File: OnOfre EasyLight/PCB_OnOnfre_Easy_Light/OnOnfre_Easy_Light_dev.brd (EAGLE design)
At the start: 44.6 x 48 mm, 38 parts, among them J3Y S8050, K1 OMRON-G3MB-202P-SSR2, K2 OMRON-G3MB-202P-SSR2, U2 esp12, X1 4P

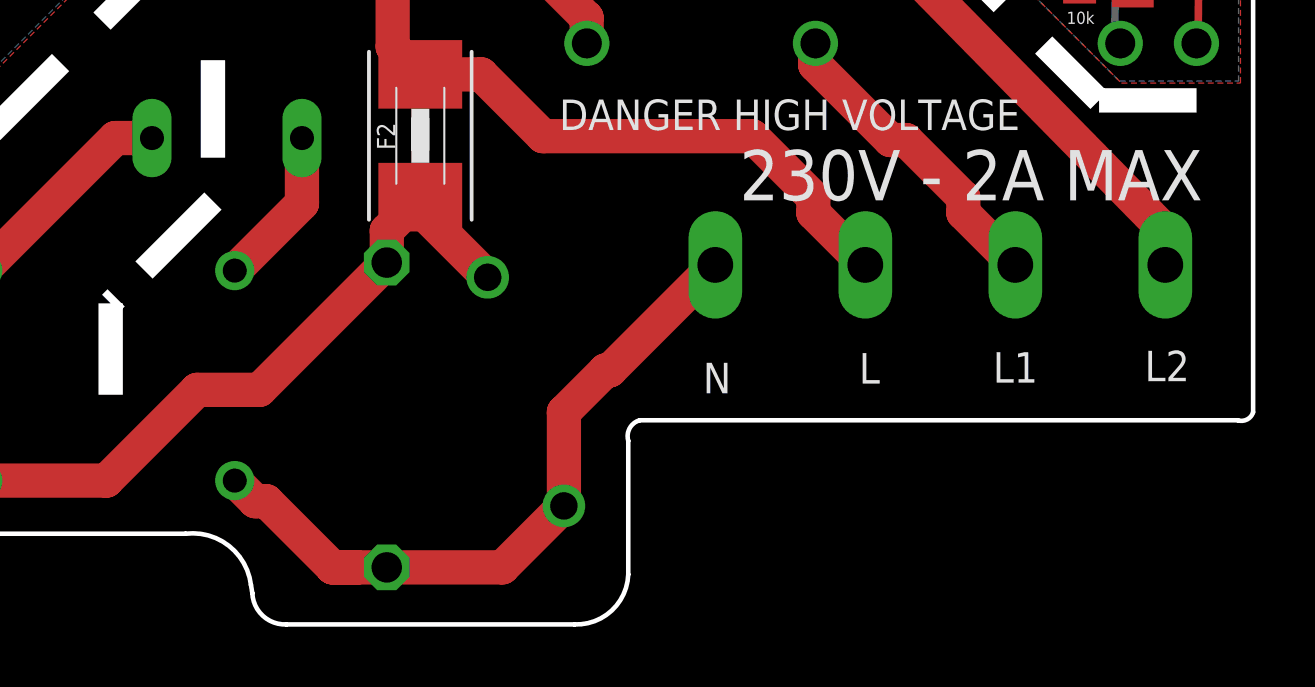
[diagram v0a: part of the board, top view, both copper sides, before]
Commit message: board
board
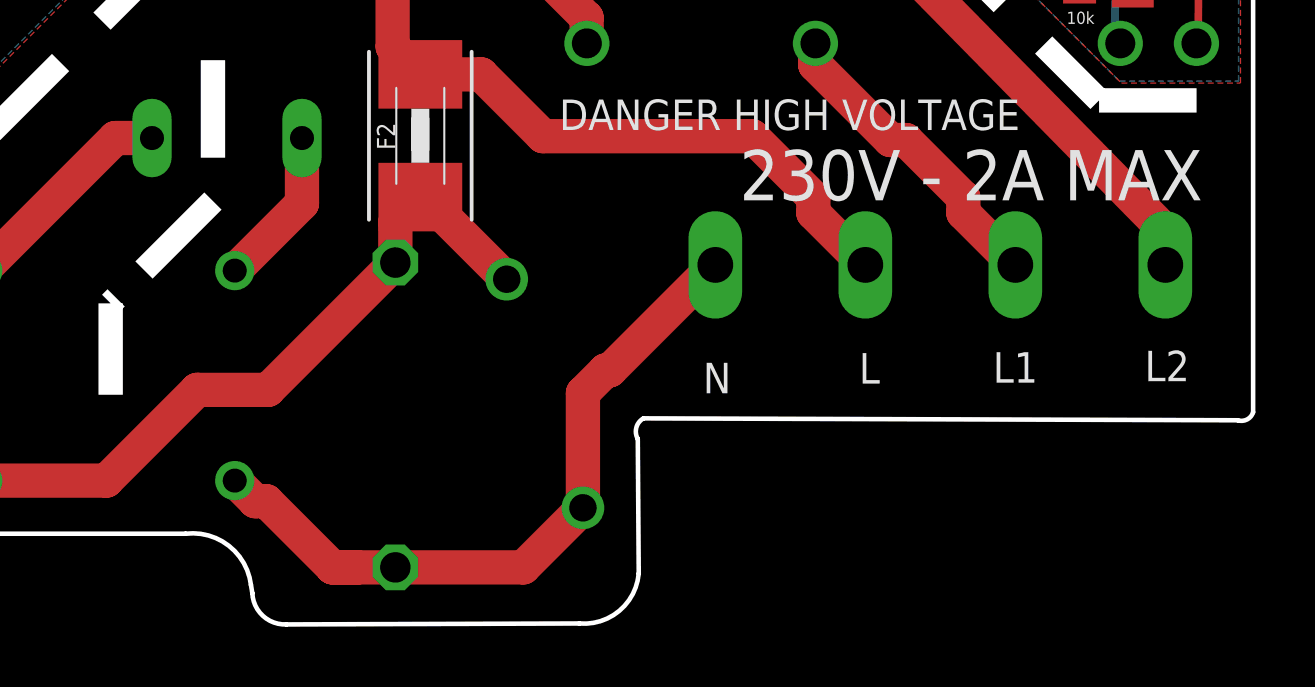
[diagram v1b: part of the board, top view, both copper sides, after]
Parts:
- moved R5 0.64 mm to (21.2, 6.26)
- moved C5 0.29 mm to (16.2, 5.54)
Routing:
- net N$2: track 22.7 -> 23.3 mm
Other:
- outline, holes or cut-outs redrawn
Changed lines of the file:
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@@
 <wire x1="11.434475" y1="-0.122359375" x2="11.48040625" y2="-0.39600625" width="0.1524" layer="20"/>
 <wire x1="11.48040625" y1="-0.39600625" x2="12.615571875" y2="-1.439584375" width="0.1524" layer="20" curve="90"/>
-<wire x1="12.615571875" y1="-1.439584375" x2="22.22130625" y2="-1.439584375" width="0.1524" layer="20"/>
-<wire x1="22.22130625" y1="-1.439584375" x2="24.011403125" y2="0.2283375" width="0.1524" layer="20" curve="90"/>
-<wire x1="24.011403125" y1="0.2283375" x2="24.011403125" y2="4.68100625" width="0.1524" layer="20"/>
-<wire x1="24.011403125" y1="4.68100625" x2="24.39040625" y2="5.365915625" width="0.1524" layer="20" curve="-90"/>
-<wire x1="24.39040625" y1="5.365915625" x2="44.32885625" y2="5.365915625" width="0.1524" layer="20"/>
+<wire x1="12.615571875" y1="-1.439584375" x2="22.38005625" y2="-1.407834375" width="0.1524" layer="20"/>
+<wire x1="22.38005625" y1="-1.407834375" x2="24.360653125" y2="0.2600875" width="0.1524" layer="20" curve="90"/>
+<wire x1="24.360653125" y1="0.2600875" x2="24.328903125" y2="4.74450625" width="0.1524" layer="20"/>
+<wire x1="24.328903125" y1="4.74450625" x2="24.51740625" y2="5.429415625" width="0.1524" layer="20" curve="-90"/>
+<wire x1="24.51740625" y1="5.429415625" x2="44.32885625" y2="5.365915625" width="0.1524" layer="20"/>
 <wire x1="44.32885625" y1="5.365915625" x2="44.839975" y2="5.632309375" width="0.1524" layer="20" curve="90"/>
 <wire x1="44.839975" y1="5.632309375" x2="44.839975" y2="27.895296875" width="0.1524" layer="20"/>
@@
 <attribute name="VALUE" x="25.457640625" y="37.142196875" size="0.4064" layer="28" rot="MR0"/>
 </element>
-<element name="R5" library="varistor" library_urn="urn:adsk.eagle:library:410" package="S07K230" package3d_urn="urn:adsk.eagle:package:30547/1" value="VARISTORS07K230" x="20.595690625" y="6.320815625" smashed="yes" rot="MR0">
-<attribute name="VALUE" x="20.895603125" y="4.746059375" size="0.4064" layer="26" rot="MR90"/>
+<element name="R5" library="varistor" library_urn="urn:adsk.eagle:library:410" package="S07K230" package3d_urn="urn:adsk.eagle:package:30547/1" value="VARISTORS07K230" x="21.230690625" y="6.257315625" smashed="yes" rot="MR0">
+<attribute name="VALUE" x="21.530603125" y="4.682559375" size="0.4064" layer="26" rot="MR90"/>
 </element>
 <element name="X1" library="con-wago-500" library_urn="urn:adsk.eagle:library:195" package="W237-4" package3d_urn="urn:adsk.eagle:package:10695/1" value="4P" x="34.4133375" y="9.27470625" smashed="yes" rot="MR180">
@@
 <attribute name="VALUE" x="21.388" y="32.326496875" size="0.4064" layer="26" ratio="10" rot="MR270"/>
 </element>
-<element name="C5" library="rcl" library_urn="urn:adsk.eagle:library:334" package="C102-054X133" package3d_urn="urn:adsk.eagle:package:23649/1" value="0.1uf 275v" x="15.961253125" y="5.54215" smashed="yes" rot="MR270">
-<attribute name="SPICEPREFIX" value="C" x="15.961253125" y="5.54215" size="1.778" layer="28" rot="MR270" display="off"/>
-<attribute name="VALUE" x="16.909746875" y="6.699475" size="0.508" layer="28" ratio="10" rot="MR270"/>
+<element name="C5" library="rcl" library_urn="urn:adsk.eagle:library:334" package="C102-054X133" package3d_urn="urn:adsk.eagle:package:23649/1" value="0.1uf 275v" x="16.247003125" y="5.54215" smashed="yes" rot="MR270">
+<attribute name="SPICEPREFIX" value="C" x="16.247003125" y="5.54215" size="1.778" layer="28" rot="MR270" display="off"/>
+<attribute name="VALUE" x="17.195496875" y="6.699475" size="0.508" layer="28" ratio="10" rot="MR270"/>
 </element>
 <element name="D1" library="diode" library_urn="urn:adsk.eagle:library:210" package="SOD323-R" package3d_urn="urn:adsk.eagle:package:43437/1" value="B5819W" x="29.011165625" y="37.9047375" smashed="yes" rot="MR270">
@@
 <wire x1="26.9133375" y1="10.54470625" x2="23.39824375" y2="7.0296125" width="1.143" layer="1"/>
 <wire x1="23.39824375" y1="7.0296125" x2="23.2560875" y2="7.0296125" width="1.143" layer="1"/>
-<wire x1="23.2560875" y1="7.0296125" x2="21.865690625" y2="5.639215625" width="1.143" layer="1"/>
-<wire x1="21.865690625" y1="5.639215625" x2="21.865690625" y2="2.510815625" width="1.143" layer="1"/>
-<wire x1="21.865690625" y1="2.510815625" x2="19.817025" y2="0.46215" width="1.143" layer="1"/>
-<wire x1="19.817025" y1="0.46215" x2="15.961253125" y2="0.46215" width="1.143" layer="1"/>
-<wire x1="15.961253125" y1="0.46215" x2="14.98990625" y2="0.46215" width="1.143" layer="1"/>
+<wire x1="23.2560875" y1="7.0296125" x2="22.500690625" y2="6.274215625" width="1.143" layer="1"/>
+<wire x1="22.500690625" y1="6.274215625" x2="22.500690625" y2="2.447315625" width="1.143" layer="1"/>
+<wire x1="22.500690625" y1="2.447315625" x2="20.515525" y2="0.46215" width="1.143" layer="1"/>
+<wire x1="20.515525" y1="0.46215" x2="16.247003125" y2="0.46215" width="1.143" layer="1"/>
+<wire x1="16.247003125" y1="0.46215" x2="14.98990625" y2="0.46215" width="1.143" layer="1"/>
 <wire x1="14.98990625" y1="0.46215" x2="14.154875" y2="0.46215" width="1.143" layer="1"/>
 <wire x1="10.894128125" y1="3.3545" x2="11.58200625" y2="2.666621875" width="1.143" layer="1"/>
@@
 <contactref element="F2" pad="2"/>
 <contactref element="L2" pad="4"/>
-<wire x1="17.07955" y1="12.8034" x2="17.07955" y2="12.37695625" width="1.143" layer="1"/>
-<wire x1="17.07955" y1="12.37695625" x2="19.325690625" y2="10.130815625" width="1.143" layer="1"/>
-<wire x1="17.07955" y1="12.8034" x2="15.961253125" y2="11.685103125" width="1.143" layer="1"/>
-<wire x1="15.961253125" y1="11.685103125" x2="15.961253125" y2="10.62215" width="1.143" layer="1"/>
-<wire x1="15.961253125" y1="10.62215" x2="11.71910625" y2="6.380003125" width="1.143" layer="1"/>
-<wire x1="11.71910625" y1="6.380003125" x2="9.640921875" y2="6.380003125" width="1.143" layer="1"/>
+<wire x1="17.22460625" y1="12.8034" x2="19.960690625" y2="10.067315625" width="1.143" layer="1"/>
+<wire x1="17.07955" y1="12.8034" x2="16.247003125" y2="11.970853125" width="1.143" layer="1"/>
+<wire x1="16.247003125" y1="11.970853125" x2="16.247003125" y2="10.62215" width="1.143" layer="1"/>
+<wire x1="16.247003125" y1="10.62215" x2="12.00485625" y2="6.380003125" width="1.143" layer="1"/>
+<wire x1="12.00485625" y1="6.380003125" x2="9.640921875" y2="6.380003125" width="1.143" layer="1"/>
 <wire x1="6.61541875" y1="3.3545" x2="2.494128125" y2="3.3545" width="1.143" layer="1"/>
 <wire x1="9.640921875" y1="6.380003125" x2="6.61541875" y2="3.3545" width="1.143" layer="1"/>
+<wire x1="17.07955" y1="12.8034" x2="17.22460625" y2="12.8034" width="1.143" layer="1"/>
 </signal>
 <signal name="EMI_NEUTRAL" class="1">
